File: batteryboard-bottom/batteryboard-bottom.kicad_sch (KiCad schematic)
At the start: 9 parts, among them J1 SFC-110-T2-X-D-A, J2 FTS-107-01-X-DV-A, U1 INA219BxD

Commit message: Updated BOMs and STEP files
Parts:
- H1, H2, H3, H4: now left out of the parts list
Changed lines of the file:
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@@
   )
   (symbol (lib_id "Mechanical:MountingHole_Pad") (at 38.354 123.317 90) (unit 1)
-    (in_bom yes) (on_board yes) (dnp no)
+    (in_bom no) (on_board yes) (dnp no)
     (property "Reference" "H1" (at 33.401 122.301 90)
       (effects (font (size 1.27 1.27)))
@@
   )
   (symbol (lib_id "Mechanical:MountingHole_Pad") (at 56.007 117.983 90) (unit 1)
-    (in_bom yes) (on_board yes) (dnp no)
+    (in_bom no) (on_board yes) (dnp no)
     (property "Reference" "H3" (at 67.564 116.713 90)
       (effects (font (size 1.27 1.27)))
@@
   )
   (symbol (lib_id "Mechanical:MountingHole_Pad") (at 56.007 123.444 90) (unit 1)
-    (in_bom yes) (on_board yes) (dnp no)
+    (in_bom no) (on_board yes) (dnp no)
     (property "Reference" "H4" (at 67.691 122.555 90)
       (effects (font (size 1.27 1.27)))
@@
   )
   (symbol (lib_id "Mechanical:MountingHole_Pad") (at 38.481 117.983 90) (unit 1)
-    (in_bom yes) (on_board yes) (dnp no)
+    (in_bom no) (on_board yes) (dnp no)
     (property "Reference" "H2" (at 33.528 116.586 90)
       (effects (font (size 1.27 1.27)))

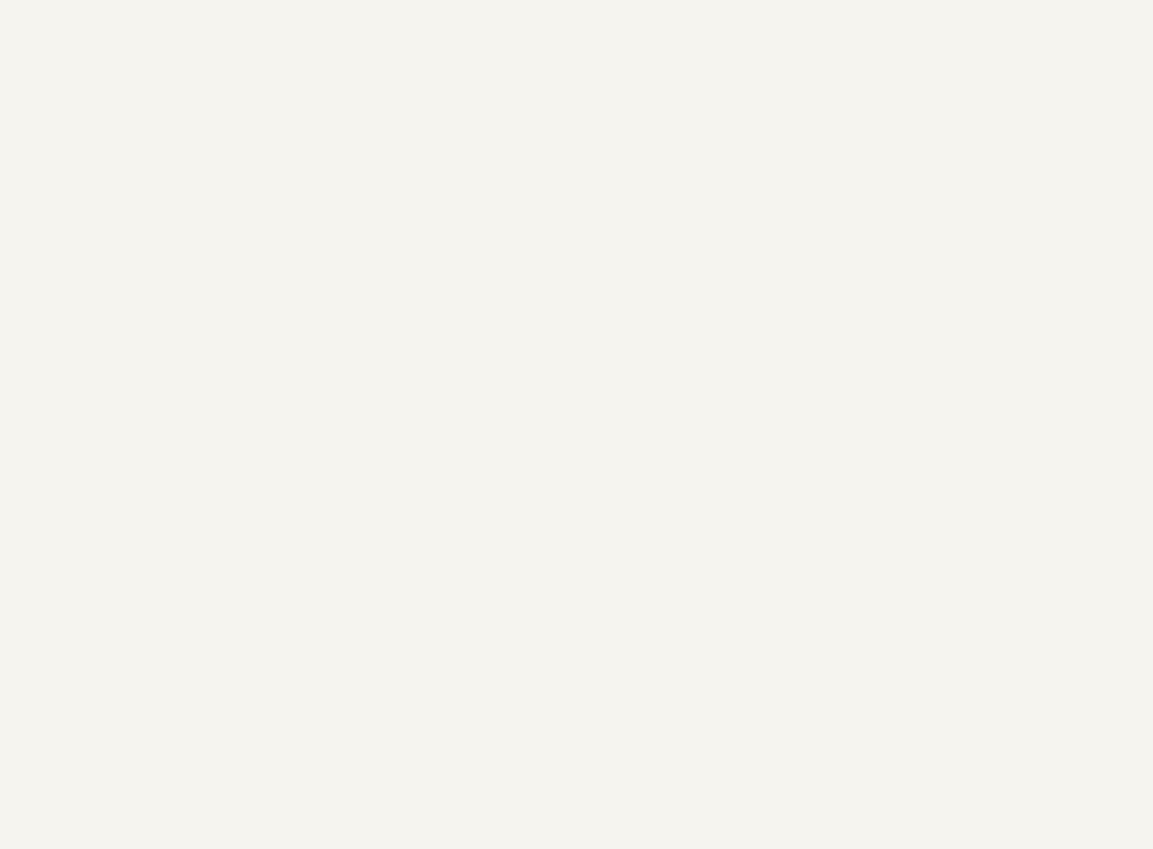
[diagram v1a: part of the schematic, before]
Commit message: Rev B3/03 updates
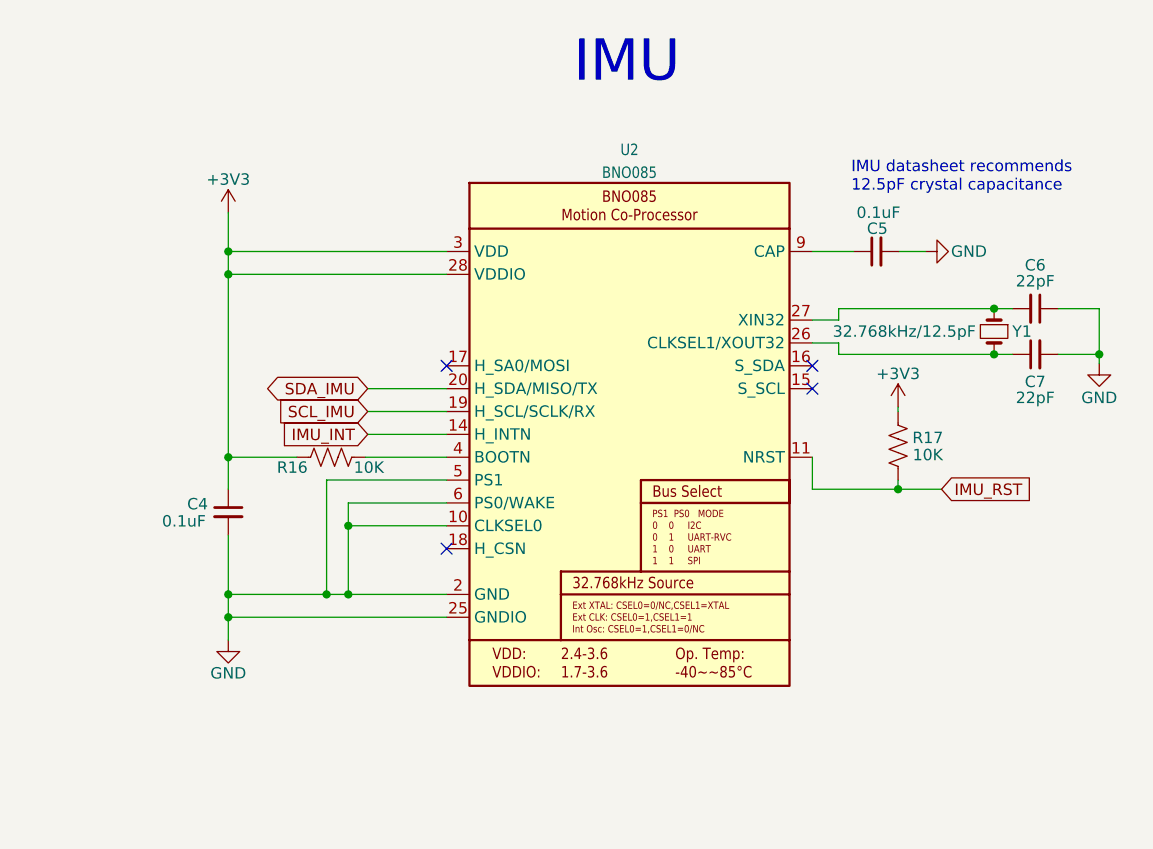
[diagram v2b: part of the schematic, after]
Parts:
- added C4, C5: 0.1uF, Capacitor_SMD:C_0603_1608Metric, symbol Device:C_Small
- added C6, C7: 22pF, Capacitor_SMD:C_0603_1608Metric, symbol Device:C_Small
- added R16, R17: 10K, Resistor_SMD:R_0603_1608Metric, symbol Device:R_US
- added U2: BNO085, mainboard:LGA-28, symbol mainboard:BNO085
- added Y1: 32.768kHz/12.5pF, Crystal:Crystal_SMD_MicroCrystal_CC7V-T1A-2Pin_3.2x1.5mm, symbol Device:Crystal_Small
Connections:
- net +3V3: now also C4.1, R16.2, R17.2, U2.28 (VDDIO), U2.3 (VDD)
- net GND: now also C4.2, C5.2, C6.1, C7.2, U2.10 (CLKSEL0), U2.2 (GND), U2.25 (GNDIO), U2.5 (PS1), U2.6 (PS0/WAKE)
- new net: C6.2, U2.27 (XIN32), Y1.1
- new net: C5.1, U2.9 (CAP)
- new net: U2.1 (NC), U2.12 (NC), U2.13 (NC), U2.21 (NC), U2.22 (NC), U2.23 (NC), U2.24 (NC), U2.7 (NC), U2.8 (NC)
- new net: C7.1, U2.26 (CLKSEL1/XOUT32), Y1.2
- new net: R16.1, U2.4 (BOOTN)
- new net IMU_INT: U2.14 (H_INTN)
- new net IMU_RST: R17.1, U2.11 (NRST)
- new net SCL_IMU: U2.19 (H_SCL/SCLK/RX)
- new net SDA_IMU: U2.20 (H_SDA/MISO/TX)
- no-connect marks 0 -> 4
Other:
- note added: "IMU"
- note added: "IMU datasheet recommends 12.5pF crystal capacitance"
